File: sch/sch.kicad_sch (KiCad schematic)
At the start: 54 parts, among them U2 PCA9548ADB, U3 MPR121QR2_BOARD, U4 MPR121QR2_BOARD, U5 MPR121QR2_BOARD, U6 ProMicro

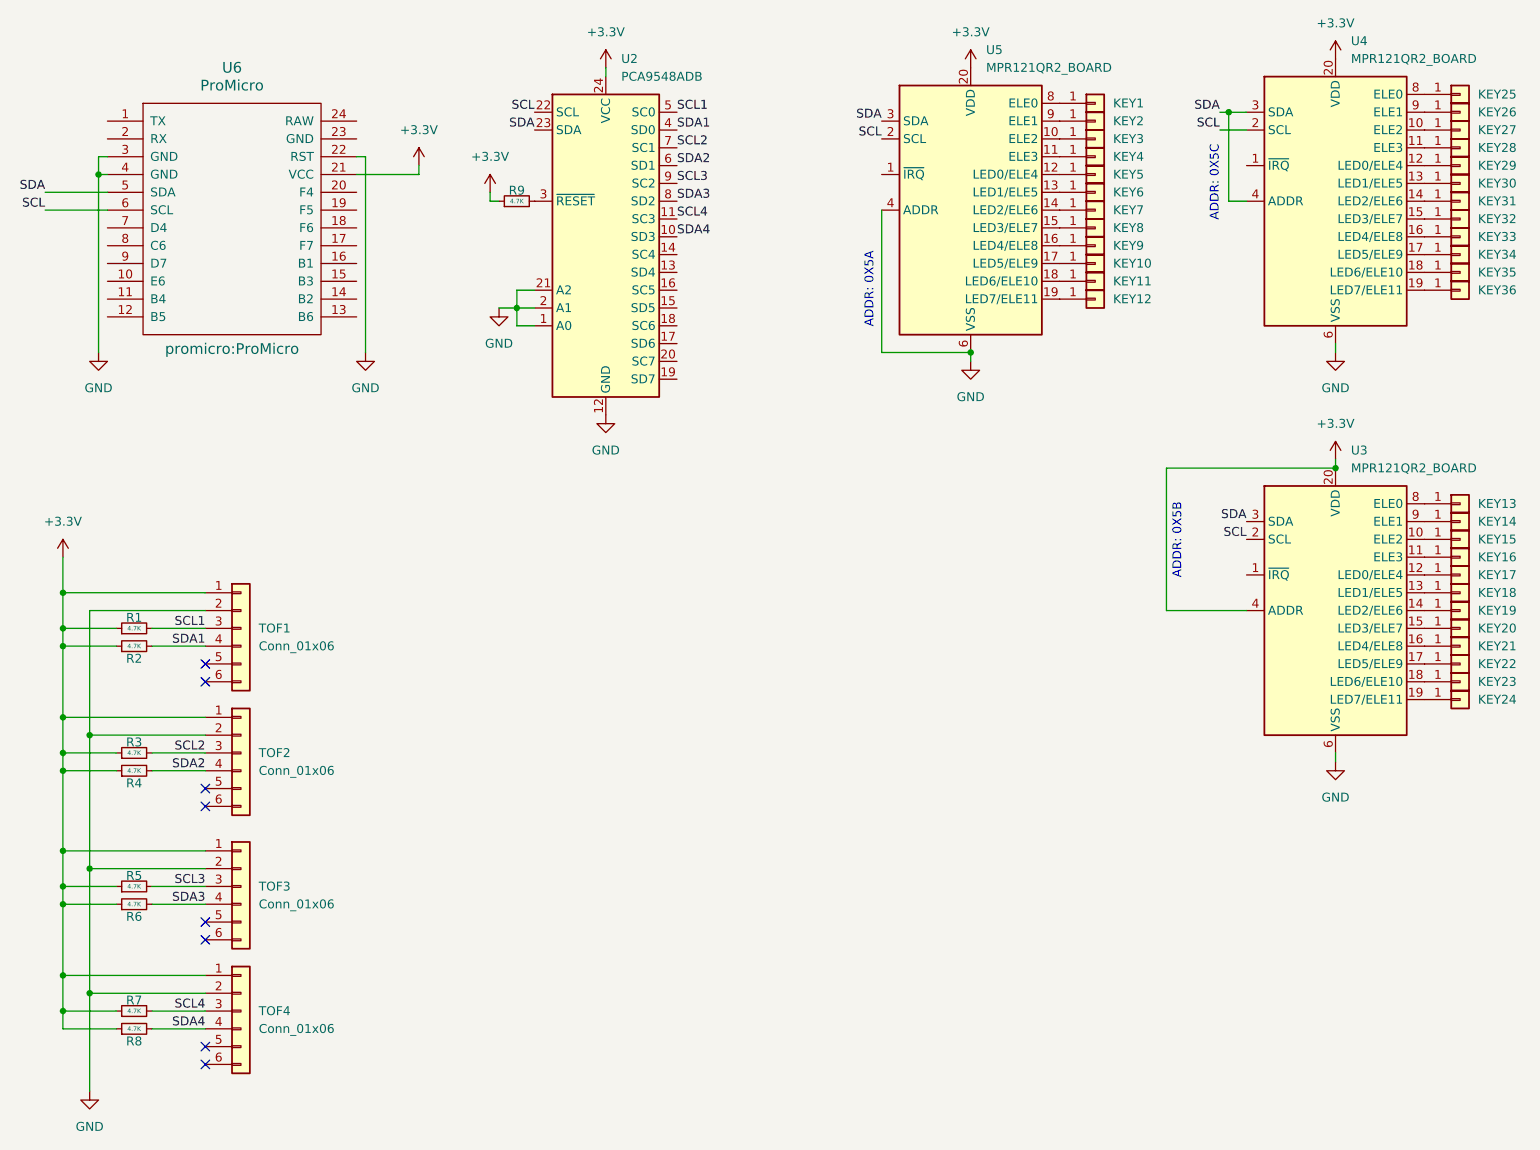
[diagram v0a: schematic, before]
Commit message: Cleaned the branch with only relevant files
It was a mess, trying to clean it up and manage the git properly
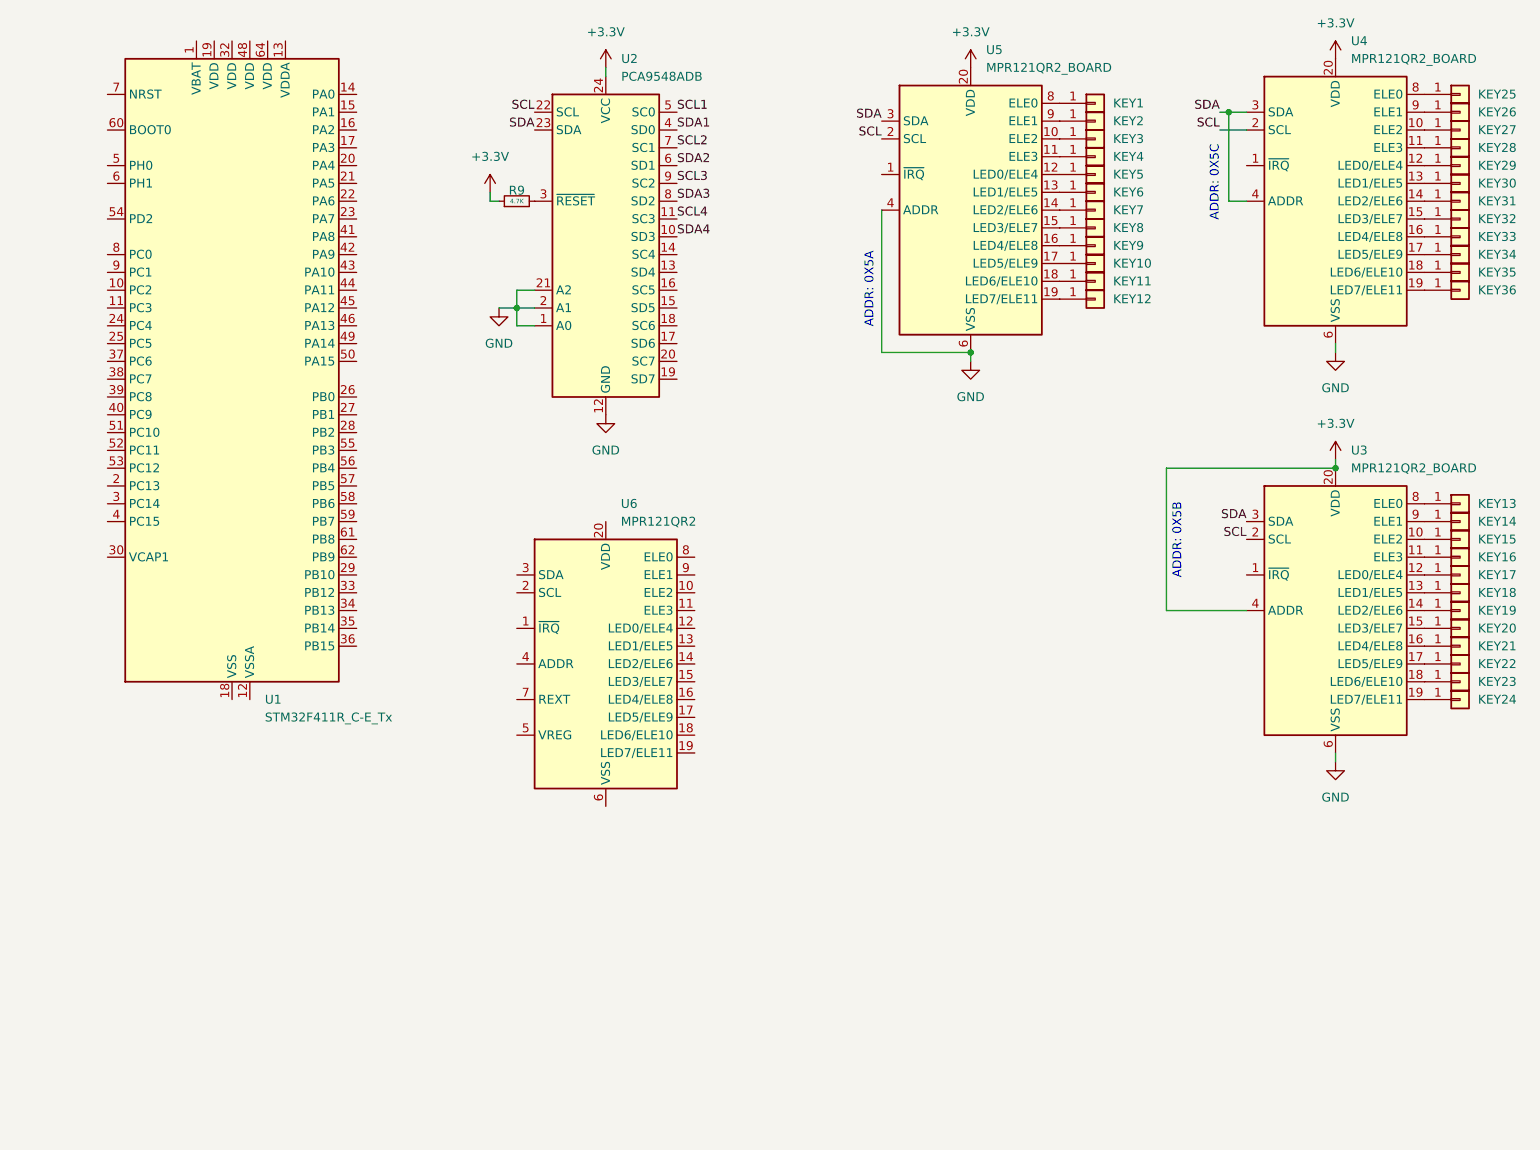
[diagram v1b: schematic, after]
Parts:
- removed R1, R2, R3, R4, R5, R6, R7, R8: 4.7K, Resistor_SMD:R_0603_1608Metric, symbol Device:R_Small
- removed TOF1, TOF2, TOF3, TOF4: Conn_01x06, Connector_PinSocket_2.54mm:PinSocket_1x06_P2.54mm_Vertical, symbol Connector_Generic:Conn_01x06
- removed U6: ProMicro, promicro:ProMicro, symbol promicro:ProMicro
- added U1: STM32F411R_C-E_Tx, Package_QFP:LQFP-64_10x10mm_P0.5mm, symbol MCU_ST_STM32F4:STM32F411R_C-E_Tx
- added U6: MPR121QR2, Package_DFN_QFN:UQFN-20_3x3mm_P0.4mm, symbol Sensor_Touch:MPR121QR2
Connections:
- new net: U1.18 (VSS), U1.31 (VSS), U1.47 (VSS), U1.63 (VSS)
- no-connect marks 8 -> 0
